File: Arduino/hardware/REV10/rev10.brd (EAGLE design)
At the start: 88.3 x 55.9 mm, 48 parts, among them IC2 ATMEGA168-AU, Q1 32768Hz, U1 TC1185SMD, U2 ARDUINO

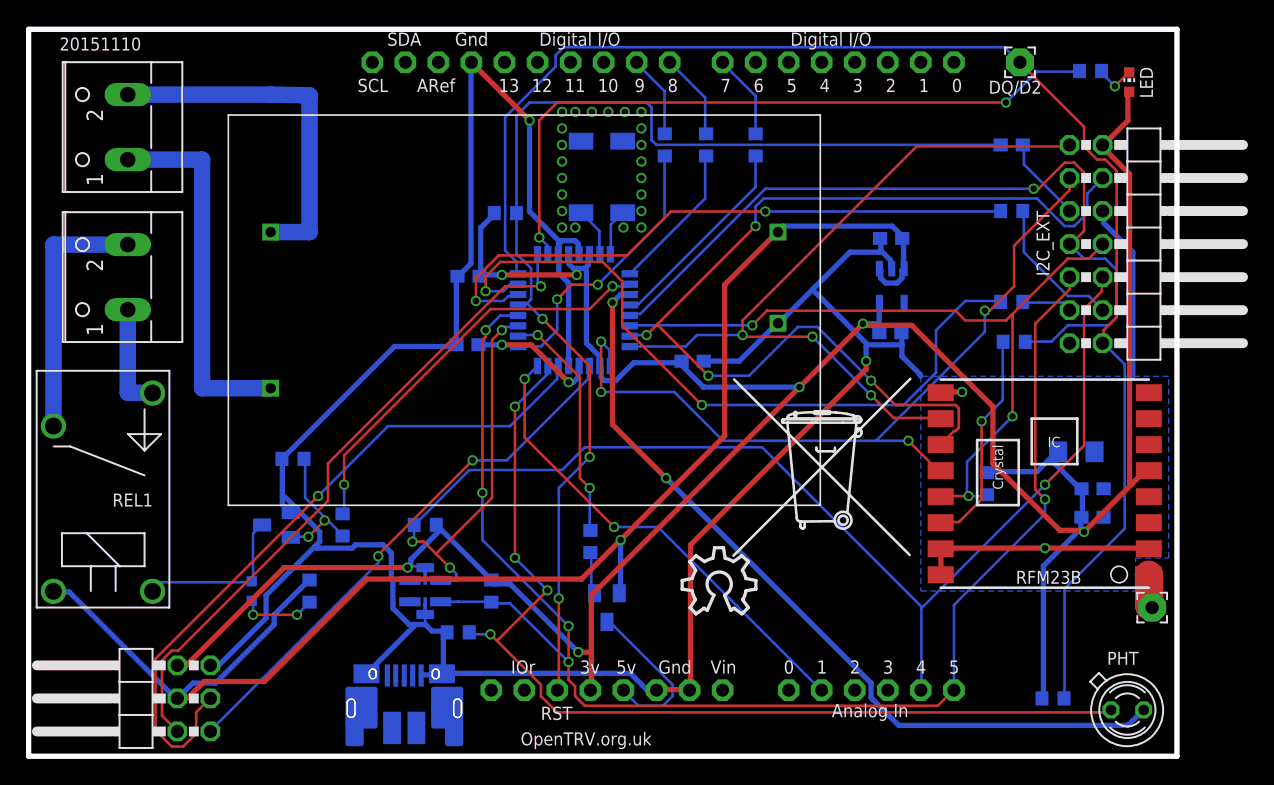
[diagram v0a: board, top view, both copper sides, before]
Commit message: rev10 touchup
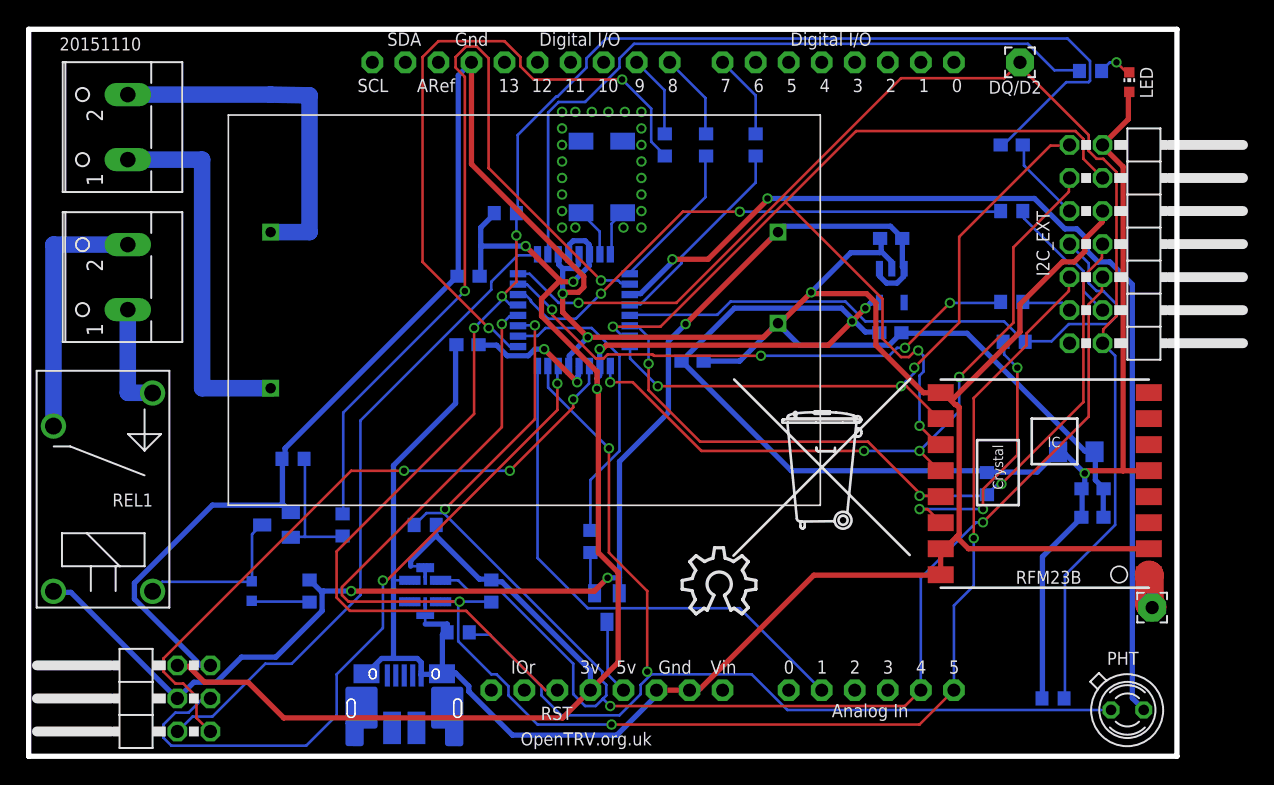
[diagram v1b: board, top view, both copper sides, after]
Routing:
- net GND: track 238.3 -> 324.8 mm, vias 4 -> 3
- net BOILER: track 31.9 -> 65.5 mm
- net RESET: track 89.0 -> 121.5 mm
- net N$11: track 21.5 -> 50.5 mm
- net VCC: track 220.0 -> 247.3 mm
- net IO_POWER_UP: track 62.5 -> 78.2 mm
- net RFM_IRQ: track 62.0 -> 47.3 mm, vias 1 -> 0
- net RX: track 55.7 -> 41.6 mm, vias 2 -> 4
- net 5V: track 115.4 -> 101.8 mm, vias 1 -> 3
- net SDA: track 113.1 -> 122.7 mm
- net SCL: track 112.6 -> 122.1 mm, vias 5 -> 4
- net N$1: track 41.7 -> 50.7 mm, vias 2 -> 3
- net D2: track 110.8 -> 102.0 mm, vias 0 -> 1
- net SPI_MISO: track 58.8 -> 51.5 mm
- net 5VGSM: track 12.5 -> 5.77 mm
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- removed copper zone on layer 16, net GND
